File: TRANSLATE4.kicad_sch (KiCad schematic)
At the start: 2 parts, among them U13 TXB0104D

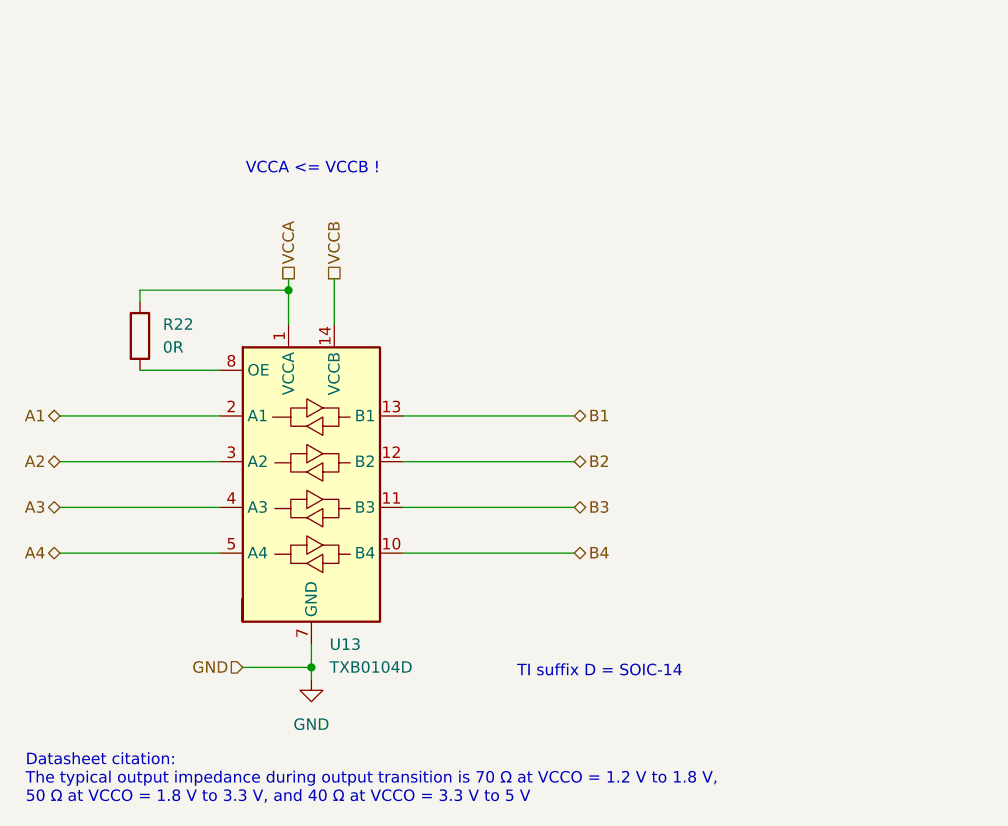
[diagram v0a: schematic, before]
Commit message: routing in progress 1
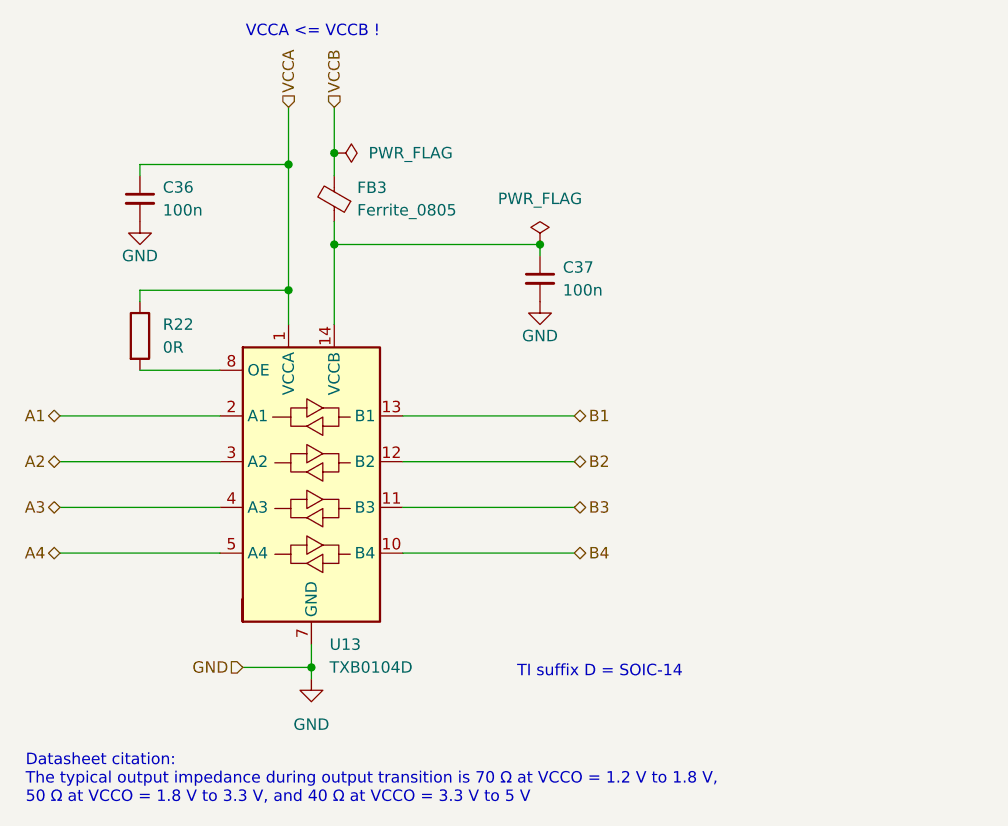
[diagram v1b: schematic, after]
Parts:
- added C36, C37: 100n, Capacitor_SMD:C_0402_1005Metric_Pad0.74x0.62mm_HandSolder, symbol Device:C_Small
- added FB3: Ferrite_0805, Resistor_SMD:R_0805_2012Metric, symbol Device:FerriteBead_Small
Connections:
- net GND: now also C36.2, C37.2
- net VCCA: now also C36.1
- net VCCB: now also FB3.2; no longer U13.14 (VCCB)
- new net: C37.1, FB3.1, U13.14 (VCCB)
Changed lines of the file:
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@@
     (comment 1 "SPI level translator 1.8V to 3.3V")
   )
+  (junction (at 135.89 45.72) (diameter 0) (color 0 0 0 0)
+  )
+  (junction (at 140.97 44.45) (diameter 0) (color 0 0 0 0)
+  )
   (junction (at 135.89 59.69) (diameter 0) (color 0 0 0 0)
   )
+  (junction (at 163.83 54.61) (diameter 0) (color 0 0 0 0)
+  )
   (junction (at 138.43 101.6) (diameter 0) (color 0 0 0 0)
   )
+  (junction (at 140.97 54.61) (diameter 0) (color 0 0 0 0)
+  )
+  (wire (pts (xy 140.97 52.07) (xy 140.97 54.61))
+    (stroke (width 0) (type default) (color 0 0 0 0))
+  )
   (wire (pts (xy 110.49 73.66) (xy 128.27 73.66))
     (stroke (width 0) (type default) (color 0 0 0 0))
@@
     (stroke (width 0) (type default) (color 0 0 0 0))
   )
-  (wire (pts (xy 135.89 59.69) (xy 135.89 58.42))
+  (wire (pts (xy 135.89 59.69) (xy 135.89 45.72))
+    (stroke (width 0) (type default) (color 0 0 0 0))
+  )
+  (wire (pts (xy 163.83 54.61) (xy 163.83 55.88))
     (stroke (width 0) (type default) (color 0 0 0 0))
   )
@@
     (stroke (width 0) (type default) (color 0 0 0 0))
   )
+  (wire (pts (xy 140.97 39.37) (xy 140.97 44.45))
+    (stroke (width 0) (type default) (color 0 0 0 0))
+  )
+  (wire (pts (xy 140.97 44.45) (xy 140.97 46.99))
+    (stroke (width 0) (type default) (color 0 0 0 0))
+  )
+  (wire (pts (xy 119.38 45.72) (xy 135.89 45.72))
+    (stroke (width 0) (type default) (color 0 0 0 0))
+  )
   (wire (pts (xy 138.43 99.06) (xy 138.43 101.6))
     (stroke (width 0) (type default) (color 0 0 0 0))
@@
     (stroke (width 0) (type default) (color 0 0 0 0))
   )
-  (wire (pts (xy 140.97 63.5) (xy 140.97 58.42))
+  (wire (pts (xy 119.38 46.99) (xy 119.38 45.72))
+    (stroke (width 0) (type default) (color 0 0 0 0))
+  )
+  (wire (pts (xy 140.97 54.61) (xy 163.83 54.61))
+    (stroke (width 0) (type default) (color 0 0 0 0))
+  )
+  (wire (pts (xy 135.89 39.37) (xy 135.89 45.72))
+    (stroke (width 0) (type default) (color 0 0 0 0))
+  )
+  (wire (pts (xy 140.97 54.61) (xy 140.97 63.5))
     (stroke (width 0) (type default) (color 0 0 0 0))
   )
@@
     (effects (font (size 1.27 1.27)) (justify left bottom))
   )
-  (text "VCCA <= VCCB !" (at 146.05 46.99 180)
+  (text "VCCA <= VCCB !" (at 146.05 31.75 180)
     (effects (font (size 1.27 1.27)) (justify right bottom))
   )
@@
     (effects (font (size 1.27 1.27)) (justify right))
   )
-  (hierarchical_label "VCCA" (shape passive) (at 135.89 58.42 90)
-    (effects (font (size 1.27 1.27)) (justify left))
-  )
-  (hierarchical_label "VCCB" (shape passive) (at 140.97 58.42 90)
+  (hierarchical_label "VCCA" (shape input) (at 135.89 39.37 90)
+    (effects (font (size 1.27 1.27)) (justify left))
+  )
+  (hierarchical_label "VCCB" (shape input) (at 140.97 39.37 90)
     (effects (font (size 1.27 1.27)) (justify left))
   )
@@
   (hierarchical_label "B1" (shape bidirectional) (at 167.64 73.66 0)
     (effects (font (size 1.27 1.27)) (justify left))
+  )
+  (symbol (lib_id "Device:C_Small") (at 119.38 49.53 0) (unit 1)
+    (in_bom yes) (on_board yes) (fields_autoplaced)
+    (property "Reference" "C36" (id 0) (at 121.92 48.2662 0)
+      (effects (font (size 1.27 1.27)) (justify left))
+    )
+    (property "Value" "100n" (id 1) (at 121.92 50.8062 0)
+      (effects (font (size 1.27 1.27)) (justify left))
+    )
+    (property "Footprint" "Capacitor_SMD:C_0402_1005Metric_Pad0.74x0.62mm_HandSolder" (id 2) (at 119.38 49.53 0)
+      (effects (font (size 1.27 1.27)) hide)
+    )
+    (property "Datasheet" "~" (id 3) (at 119.38 49.53 0)
+      (effects (font (size 1.27 1.27)) hide)
+    )
+    (pin "1")
+    (pin "2")
   )
   (symbol (lib_id "power:GND") (at 138.43 102.87 0) (unit 1)
@@
     )
     (pin "1")
+  )
+  (symbol (lib_id "Device:FerriteBead_Small") (at 140.97 49.53 180) (unit 1)
+    (in_bom yes) (on_board yes)
+    (property "Reference" "FB3" (id 0) (at 143.51 48.298 0)
+      (effects (font (size 1.27 1.27)) (justify right))
+    )
+    (property "Value" "Ferrite_0805" (id 1) (at 143.51 50.8 0)
+      (effects (font (size 1.27 1.27)) (justify right))
+    )
+    (property "Footprint" "Resistor_SMD:R_0805_2012Metric" (id 2) (at 142.748 49.53 90)
+      (effects (font (size 1.27 1.27)) hide)
+    )
+    (property "Datasheet" "~" (id 3) (at 140.97 49.53 0)
+      (effects (font (size 1.27 1.27)) hide)
+    )
+    (pin "1")
+    (pin "2")
   )
   (symbol (lib_id "Device:R") (at 119.38 64.77 0) (unit 1)
@@
     (pin "9")
   )
+  (symbol (lib_id "Device:C_Small") (at 163.83 58.42 0) (unit 1)
+    (in_bom yes) (on_board yes) (fields_autoplaced)
+    (property "Reference" "C37" (id 0) (at 166.37 57.1562 0)
+      (effects (font (size 1.27 1.27)) (justify left))
+    )
+    (property "Value" "100n" (id 1) (at 166.37 59.6962 0)
+      (effects (font (size 1.27 1.27)) (justify left))
+    )
+    (property "Footprint" "Capacitor_SMD:C_0402_1005Metric_Pad0.74x0.62mm_HandSolder" (id 2) (at 163.83 58.42 0)
+      (effects (font (size 1.27 1.27)) hide)
+    )
+    (property "Datasheet" "~" (id 3) (at 163.83 58.42 0)
+      (effects (font (size 1.27 1.27)) hide)
+    )
+    (pin "1")
+    (pin "2")
+  )
+  (symbol (lib_id "power:PWR_FLAG") (at 163.83 54.61 0) (unit 1)
+    (in_bom yes) (on_board yes) (fields_autoplaced)
+    (property "Reference" "#FLG0103" (id 0) (at 163.83 52.705 0)
+      (effects (font (size 1.27 1.27)) hide)
+    )
+    (property "Value" "PWR_FLAG" (id 1) (at 163.83 49.53 0))
+    (property "Footprint" "" (id 2) (at 163.83 54.61 0)
+      (effects (font (size 1.27 1.27)) hide)
+    )
+    (property "Datasheet" "~" (id 3) (at 163.83 54.61 0)
+      (effects (font (size 1.27 1.27)) hide)
+    )
+    (pin "1")
+  )
+  (symbol (lib_id "power:GND") (at 163.83 60.96 0) (unit 1)
+    (in_bom yes) (on_board yes)
+    (property "Reference" "#PWR0145" (id 0) (at 163.83 67.31 0)
+      (effects (font (size 1.27 1.27)) hide)
+    )
+    (property "Value" "GND" (id 1) (at 163.83 64.77 0))
+    (property "Footprint" "" (id 2) (at 163.83 60.96 0)
+      (effects (font (size 1.27 1.27)) hide)
+    )
+    (property "Datasheet" "" (id 3) (at 163.83 60.96 0)
+      (effects (font (size 1.27 1.27)) hide)
+    )
+    (pin "1")
+  )
+  (symbol (lib_id "power:PWR_FLAG") (at 140.97 44.45 270) (unit 1)
+    (in_bom yes) (on_board yes) (fields_autoplaced)
+    (property "Reference" "#FLG0104" (id 0) (at 142.875 44.45 0)
+      (effects (font (size 1.27 1.27)) hide)
+    )
+    (property "Value" "PWR_FLAG" (id 1) (at 144.78 44.4499 90)
+      (effects (font (size 1.27 1.27)) (justify left))
+    )
+    (property "Footprint" "" (id 2) (at 140.97 44.45 0)
+      (effects (font (size 1.27 1.27)) hide)
+    )
+    (property "Datasheet" "~" (id 3) (at 140.97 44.45 0)
+      (effects (font (size 1.27 1.27)) hide)
+    )
+    (pin "1")
+  )
+  (symbol (lib_id "power:GND") (at 119.38 52.07 0) (unit 1)
+    (in_bom yes) (on_board yes)
+    (property "Reference" "#PWR0144" (id 0) (at 119.38 58.42 0)
+      (effects (font (size 1.27 1.27)) hide)
+    )
+    (property "Value" "GND" (id 1) (at 119.38 55.88 0))
+    (property "Footprint" "" (id 2) (at 119.38 52.07 0)
+      (effects (font (size 1.27 1.27)) hide)
+    )
+    (property "Datasheet" "" (id 3) (at 119.38 52.07 0)
+      (effects (font (size 1.27 1.27)) hide)
+    )
+    (pin "1")
+  )
 )
